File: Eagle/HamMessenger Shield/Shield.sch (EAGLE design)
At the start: 23 parts, among them J2 KEYBOARD GROVE, M1 ARDUINO-PRO-MINI-3.3V, Q3 MOSFET-NCHANNEL2N7002PW

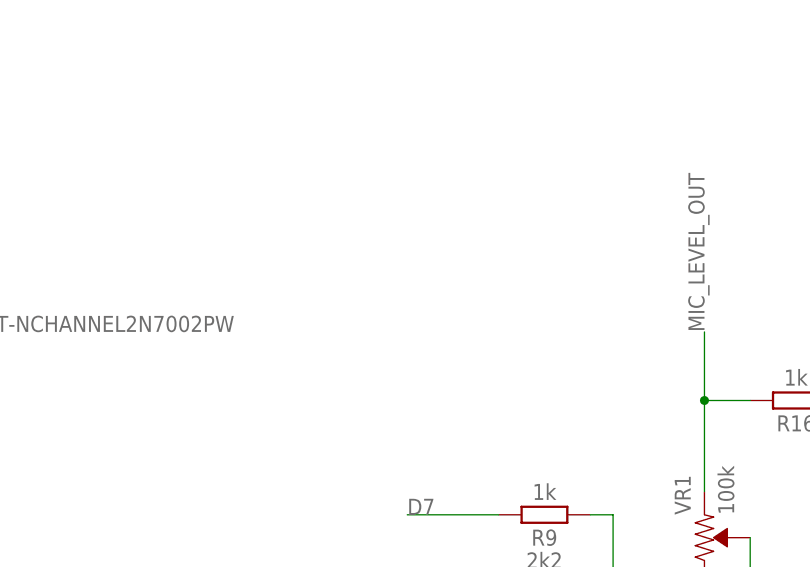
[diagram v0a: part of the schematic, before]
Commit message: PCB Updates
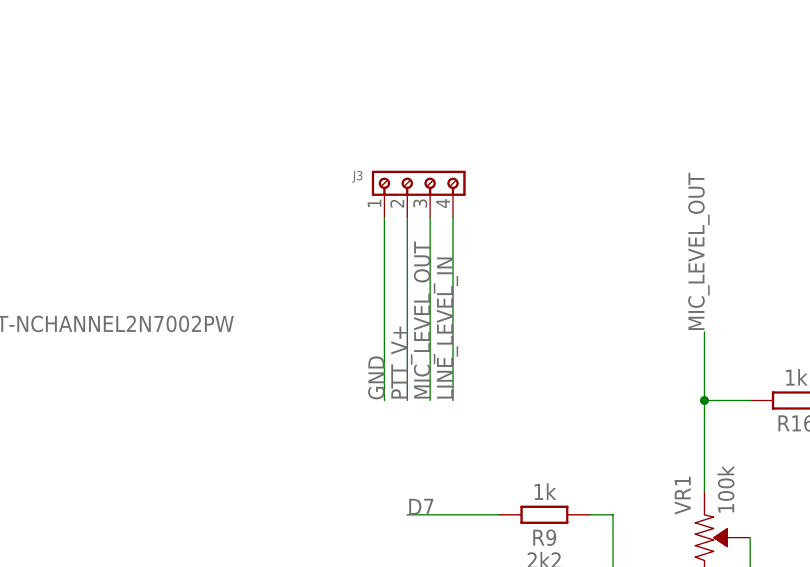
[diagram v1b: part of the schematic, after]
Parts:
- added J3: (no value), Wurth_Connectors_WR-TBL Rising Cage Clamp:691210910004
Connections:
- net GND: now also J3.1
- net LINE_LEVEL_IN: now also J3.4
- net MIC_LEVEL_OUT: now also J3.3
- net PTT_V+: now also J3.2
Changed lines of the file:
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@@
 <part name="C3" library="Capacitor" library_urn="urn:adsk.eagle:library:16290819" deviceset="C" device="CHIP-0805(2012-METRIC)" package3d_urn="urn:adsk.eagle:package:16290897/2" technology="_" value="100nf"/>
 <part name="C1" library="adafruit" library_urn="urn:adsk.eagle:library:420" deviceset="CPOL-US" device="CT3528" package3d_urn="urn:adsk.eagle:package:6240405/1" value="4.7uf"/>
+<part name="J3" library="Wurth_Connectors_WR-TBL Rising Cage Clamp" library_urn="urn:adsk.eagle:library:16280519" deviceset="691210910004" device="" package3d_urn="urn:adsk.eagle:package:16248430/2"/>
 </parts>
 <sheets>
@@
 <attribute name="VALUE" x="158.496" y="36.449" size="1.778" layer="96"/>
 </instance>
+<instance part="J3" gate="G$1" x="127" y="93.98" smashed="yes">
+<attribute name="NAME" x="119.58" y="93.058" size="1.016" layer="95" align="bottom-right"/>
+<attribute name="VALUE" x="119.63" y="91.4" size="1.016" layer="96" align="bottom-right"/>
+</instance>
 </instances>
 <busses>
@@
 <wire x1="162.56" y1="68.58" x2="157.48" y2="68.58" width="0.1524" layer="91"/>
 <junction x="157.48" y="68.58"/>
+</segment>
+<segment>
+<pinref part="J3" gate="G$1" pin="3"/>
+<wire x1="127" y1="88.9" x2="127" y2="68.58" width="0.1524" layer="91"/>
+<label x="127" y="68.58" size="1.778" layer="95" rot="R90"/>
 </segment>
 </net>
@@
 <junction x="175.26" y="15.24"/>
 </segment>
+<segment>
+<pinref part="J3" gate="G$1" pin="1"/>
+<wire x1="121.92" y1="88.9" x2="121.92" y2="68.58" width="0.1524" layer="91"/>
+<label x="121.92" y="68.58" size="1.778" layer="95" rot="R90"/>
+</segment>
 </net>
 <net name="LINE_LEVEL_IN" class="0">
@@
 <pinref part="C4" gate="G$1" pin="2"/>
 <label x="93.98" y="27.94" size="1.778" layer="95"/>
+</segment>
+<segment>
+<pinref part="J3" gate="G$1" pin="4"/>
+<wire x1="129.54" y1="88.9" x2="129.54" y2="68.58" width="0.1524" layer="91"/>
+<label x="129.54" y="68.58" size="1.778" layer="95" rot="R90"/>
 </segment>
 </net>
@@
 <label x="66.04" y="86.36" size="1.778" layer="95"/>
 </segment>
-</net>
+<segment>
+<pinref part="J3" gate="G$1" pin="2"/>
+<wire x1="124.46" y1="88.9" x2="124.46" y2="68.58" width="0.1524" layer="91"/>
+<label x="124.46" y="68.58" size="1.778" layer="95" rot="R90"/>
+</segment>
+</net>
